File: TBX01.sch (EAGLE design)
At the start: 75 parts, among them IC1 TPS62120, SW1 SW-TACTILE-PTS840P, SW2 SW-TACTILE-PTS840P, SW3 SW-TACTILE-PTS840P, SW4 SW-TACTILE-PTS840P, U3 STM32L151CCT6, U6 MCP73833, X2 FH12-10S-0.5SH, Y1 CRYSTAL.ABS07

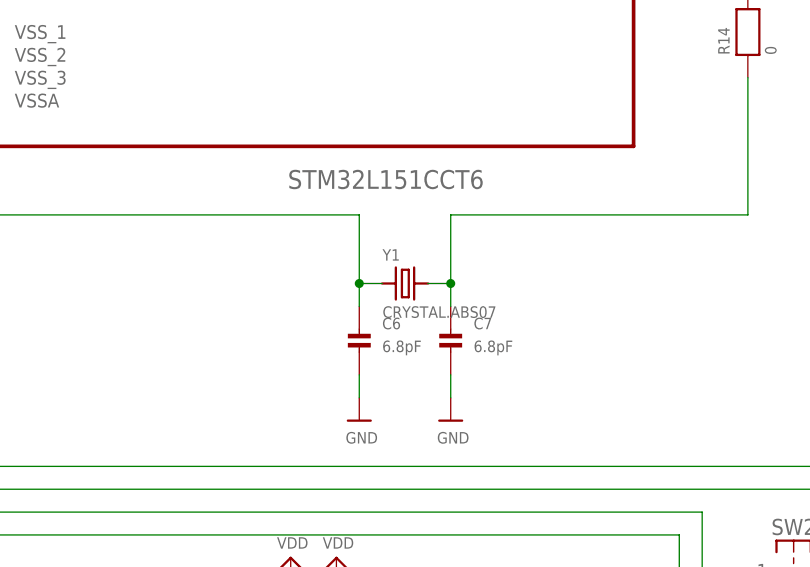
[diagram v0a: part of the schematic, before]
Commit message: TBX01 v0.2-r201508171545
On branch master
	.~lock.TBX-01_power.ods#
nothing added to commit but untracked files present (use "git add" to track)
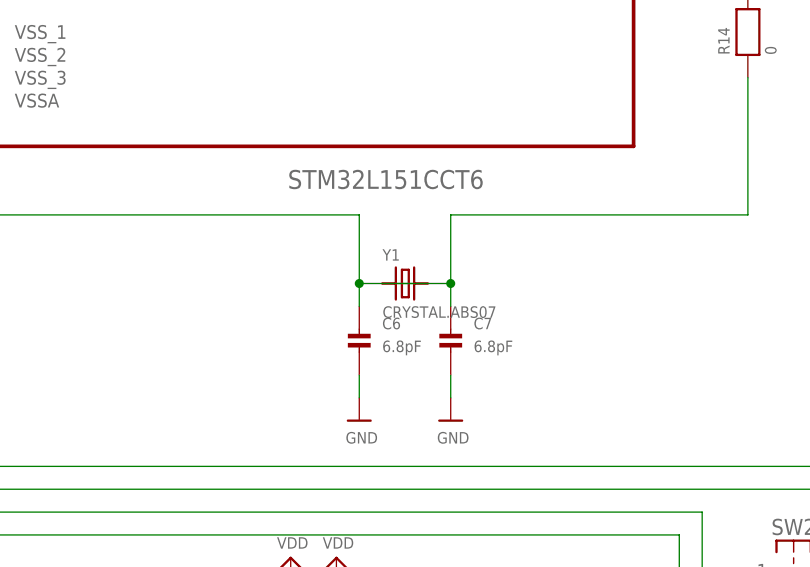
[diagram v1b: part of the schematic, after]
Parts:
- D1: device microbuilder:DIODESMA -> microbuilder:DIODESOD-123
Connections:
- net N$18: now also Y1.2; no longer Y1.1
- net N$22: now also Y1.1; no longer Y1.2
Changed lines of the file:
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@@
 <part name="R22" library="microbuilder" deviceset="RESISTOR" device="0603" value="4.7k"/>
 <part name="R23" library="microbuilder" deviceset="RESISTOR" device="0603" value="4.7k"/>
-<part name="D1" library="microbuilder" deviceset="DIODE" device="SMA"/>
+<part name="D1" library="microbuilder" deviceset="DIODE" device="SOD-123"/>
 </parts>
 <sheets>
@@
 <wire x1="-38.1" y1="10.16" x2="-38.1" y2="2.54" width="0.1524" layer="91"/>
 <pinref part="C6" gate="G$1" pin="P$1"/>
-<pinref part="Y1" gate="G$1" pin="1"/>
+<pinref part="Y1" gate="G$1" pin="2"/>
 <wire x1="-38.1" y1="2.54" x2="-38.1" y2="0" width="0.1524" layer="91"/>
-<wire x1="-38.1" y1="2.54" x2="-35.56" y2="2.54" width="0.1524" layer="91"/>
+<wire x1="-38.1" y1="2.54" x2="-30.48" y2="2.54" width="0.1524" layer="91"/>
 <junction x="-38.1" y="2.54"/>
 </segment>
@@
 <pinref part="C7" gate="G$1" pin="P$1"/>
 <wire x1="-27.94" y1="2.54" x2="-27.94" y2="0" width="0.1524" layer="91"/>
-<pinref part="Y1" gate="G$1" pin="2"/>
-<wire x1="-30.48" y1="2.54" x2="-27.94" y2="2.54" width="0.1524" layer="91"/>
+<pinref part="Y1" gate="G$1" pin="1"/>
+<wire x1="-35.56" y1="2.54" x2="-27.94" y2="2.54" width="0.1524" layer="91"/>
 <junction x="-27.94" y="2.54"/>
 <wire x1="5.08" y1="25.4" x2="5.08" y2="10.16" width="0.1524" layer="91"/>

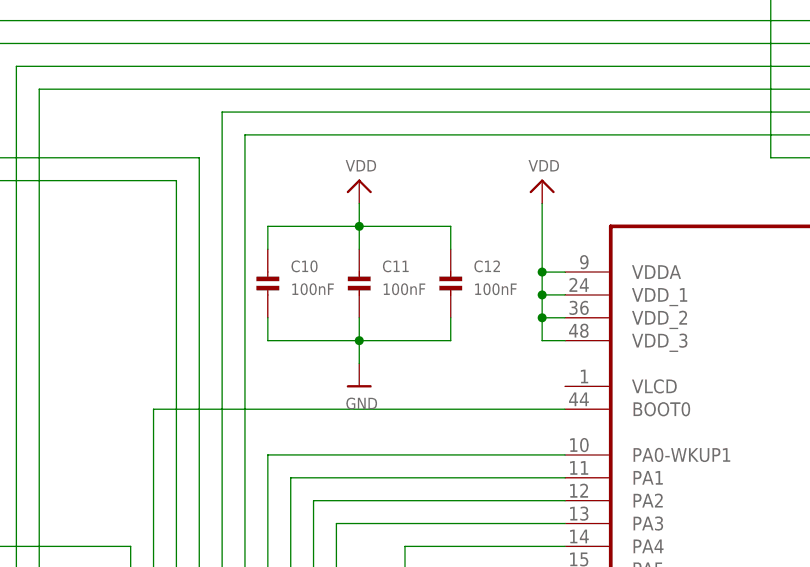
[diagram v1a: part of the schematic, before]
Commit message: TBX01 v0.2-r201508172343
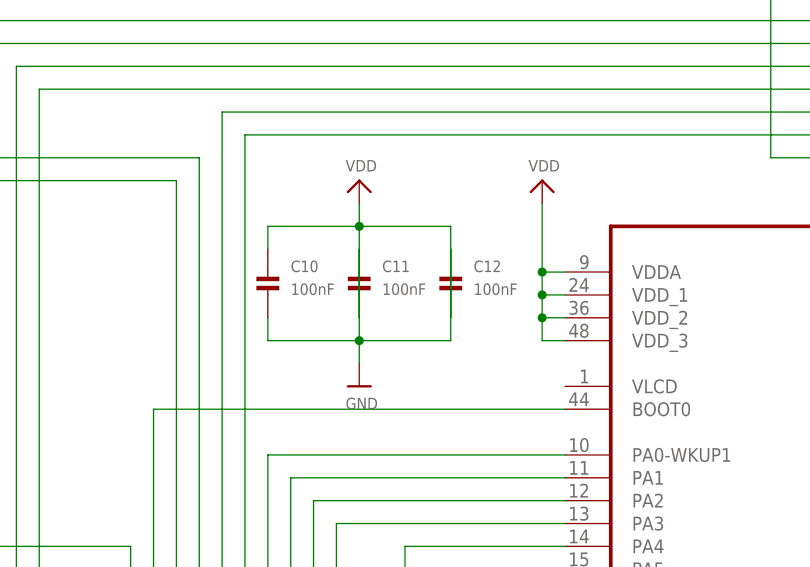
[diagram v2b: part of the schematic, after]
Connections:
- net GND: now also C11.P$1, C12.P$1; no longer C11.P$2, C12.P$2
- net VDD: now also C11.P$2, C12.P$2; no longer C11.P$1, C12.P$1
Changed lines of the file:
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@@
 <pinref part="C10" gate="G$1" pin="P$2"/>
 <wire x1="-116.84" y1="93.98" x2="-116.84" y2="91.44" width="0.1524" layer="91"/>
-<pinref part="C11" gate="G$1" pin="P$2"/>
+<pinref part="C11" gate="G$1" pin="P$1"/>
 <wire x1="-116.84" y1="91.44" x2="-106.68" y2="91.44" width="0.1524" layer="91"/>
-<wire x1="-106.68" y1="91.44" x2="-106.68" y2="93.98" width="0.1524" layer="91"/>
-<pinref part="C12" gate="G$1" pin="P$2"/>
+<wire x1="-106.68" y1="91.44" x2="-106.68" y2="101.6" width="0.1524" layer="91"/>
+<pinref part="C12" gate="G$1" pin="P$1"/>
 <wire x1="-106.68" y1="91.44" x2="-96.52" y2="91.44" width="0.1524" layer="91"/>
-<wire x1="-96.52" y1="91.44" x2="-96.52" y2="93.98" width="0.1524" layer="91"/>
+<wire x1="-96.52" y1="91.44" x2="-96.52" y2="101.6" width="0.1524" layer="91"/>
 <junction x="-106.68" y="91.44"/>
 <pinref part="U$29" gate="G$1" pin="GND"/>
@@
 </segment>
 <segment>
-<pinref part="C11" gate="G$1" pin="P$1"/>
+<pinref part="C11" gate="G$1" pin="P$2"/>
 <pinref part="U$27" gate="G$1" pin="VDD"/>
-<wire x1="-106.68" y1="101.6" x2="-106.68" y2="104.14" width="0.1524" layer="91"/>
-<pinref part="C12" gate="G$1" pin="P$1"/>
+<wire x1="-106.68" y1="93.98" x2="-106.68" y2="104.14" width="0.1524" layer="91"/>
+<pinref part="C12" gate="G$1" pin="P$2"/>
 <wire x1="-106.68" y1="104.14" x2="-106.68" y2="106.68" width="0.1524" layer="91"/>
-<wire x1="-96.52" y1="101.6" x2="-96.52" y2="104.14" width="0.1524" layer="91"/>
+<wire x1="-96.52" y1="93.98" x2="-96.52" y2="104.14" width="0.1524" layer="91"/>
 <wire x1="-96.52" y1="104.14" x2="-106.68" y2="104.14" width="0.1524" layer="91"/>
 <junction x="-106.68" y="104.14"/>

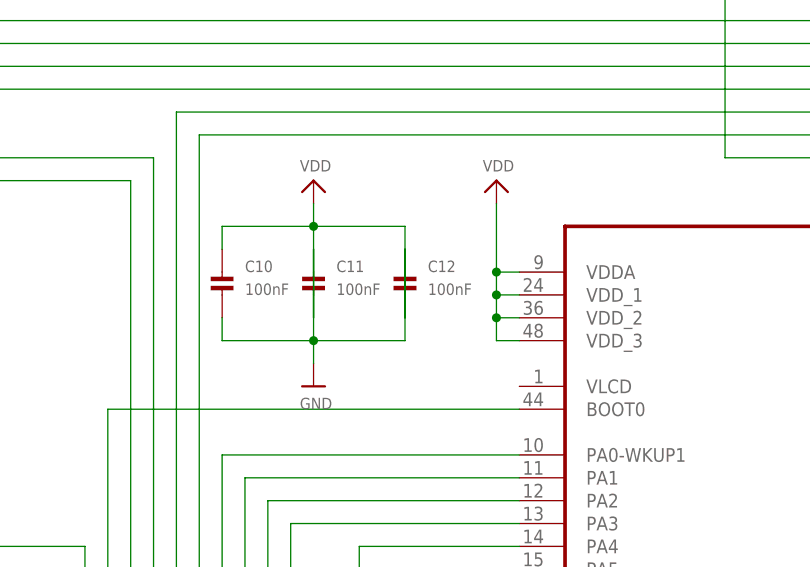
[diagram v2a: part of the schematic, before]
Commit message: TBX01 v0.2-r201508181630
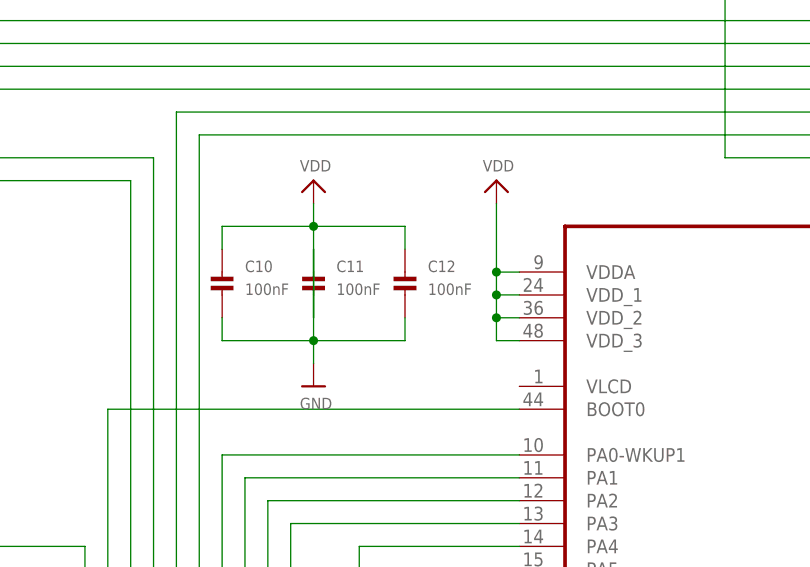
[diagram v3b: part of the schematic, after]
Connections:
- net GND: now also C12.P$2; no longer C12.P$1
- net VDD: now also C12.P$1; no longer C12.P$2
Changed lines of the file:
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@@
 <wire x1="-116.84" y1="91.44" x2="-106.68" y2="91.44" width="0.1524" layer="91"/>
 <wire x1="-106.68" y1="91.44" x2="-106.68" y2="101.6" width="0.1524" layer="91"/>
-<pinref part="C12" gate="G$1" pin="P$1"/>
+<pinref part="C12" gate="G$1" pin="P$2"/>
 <wire x1="-106.68" y1="91.44" x2="-96.52" y2="91.44" width="0.1524" layer="91"/>
-<wire x1="-96.52" y1="91.44" x2="-96.52" y2="101.6" width="0.1524" layer="91"/>
+<wire x1="-96.52" y1="91.44" x2="-96.52" y2="93.98" width="0.1524" layer="91"/>
 <junction x="-106.68" y="91.44"/>
 <pinref part="U$29" gate="G$1" pin="GND"/>
@@
 <pinref part="U$27" gate="G$1" pin="VDD"/>
 <wire x1="-106.68" y1="93.98" x2="-106.68" y2="104.14" width="0.1524" layer="91"/>
-<pinref part="C12" gate="G$1" pin="P$2"/>
+<pinref part="C12" gate="G$1" pin="P$1"/>
 <wire x1="-106.68" y1="104.14" x2="-106.68" y2="106.68" width="0.1524" layer="91"/>
-<wire x1="-96.52" y1="93.98" x2="-96.52" y2="104.14" width="0.1524" layer="91"/>
+<wire x1="-96.52" y1="101.6" x2="-96.52" y2="104.14" width="0.1524" layer="91"/>
 <wire x1="-96.52" y1="104.14" x2="-106.68" y2="104.14" width="0.1524" layer="91"/>
 <junction x="-106.68" y="104.14"/>
